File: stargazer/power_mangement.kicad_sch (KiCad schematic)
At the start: 32 parts, among them J1 1935161, J2 10118193-0001LF, J3 Conn_01x02_Pin, J4 1935161, SW1 JS202011SCQN, U1 ESP32-C3-WROOM-02U-N4, U2 MCP73831-2-OT, U3 USBLC6-2SC6, U4 LM66100DCKR, U5 LM66100DCKR, U6 AP2112K-3.3

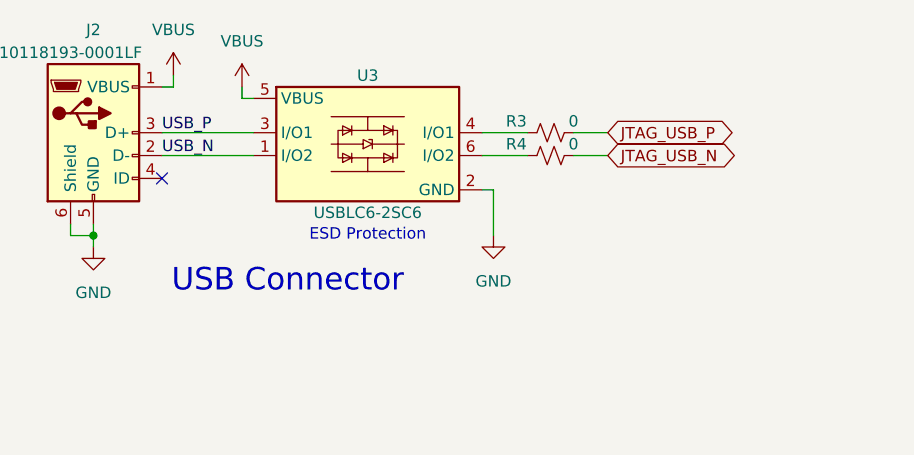
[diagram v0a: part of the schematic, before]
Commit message: Revision B
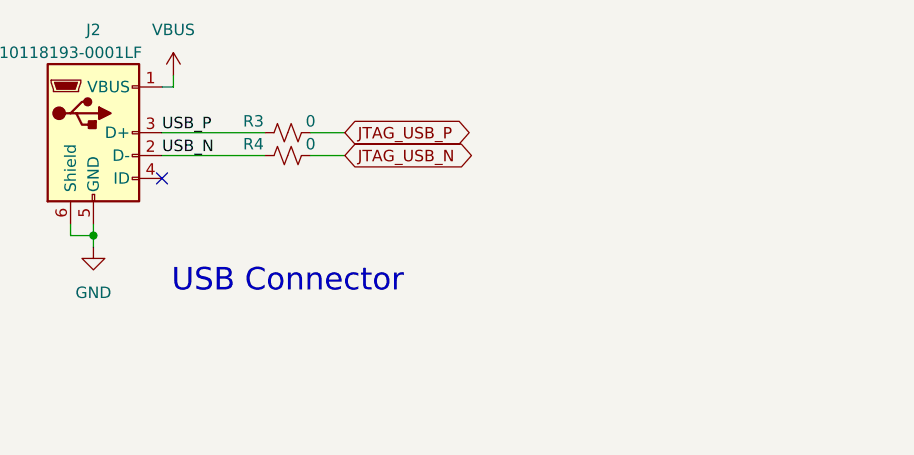
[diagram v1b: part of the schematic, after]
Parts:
- removed U3: USBLC6-2SC6, Package_TO_SOT_SMD:SOT-23-6, symbol MCU:USBLC6-2SC6
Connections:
- net USB_N: now also R4.1
- net USB_P: now also R3.1
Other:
- note removed: "ESD Protection"
- moved on the sheet: R3, R4
